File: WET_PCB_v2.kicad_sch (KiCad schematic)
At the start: 0 parts

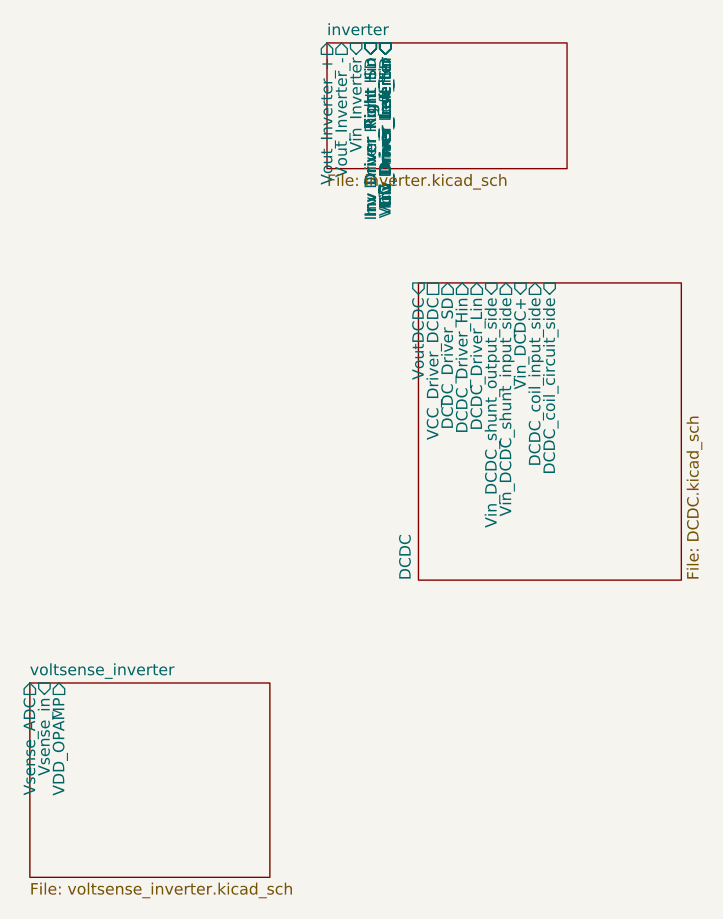
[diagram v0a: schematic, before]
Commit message: Autosave
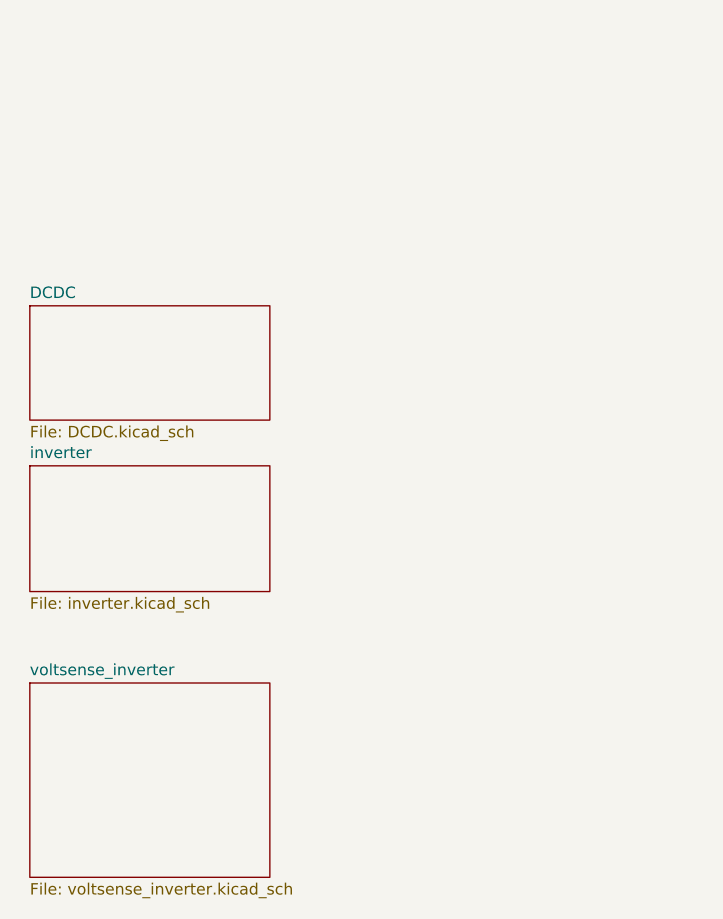
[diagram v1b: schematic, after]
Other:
- sheet DCDC ports: added none; removed DCDC_Driver_Hin, DCDC_Driver_Lin, DCDC_Driver_SD, DCDC_coil_circuit_side, DCDC_coil_input_side, VCC_Driver_DCDC, Vin_DCDC+, Vin_DCDC_shunt_input_side, Vin_DCDC_shunt_output_side, VoutDCDC
- sheet inverter ports: added none; removed Inv_Driver_Left_Hin, Inv_Driver_Left_Lin, Inv_Driver_Left_SD, Inv_Driver_Right_Hin, Inv_Driver_Right_Lin, Inv_Driver_Right_SD, VCC_Driver_Inverter, VDD_Driver_Inverter, Vin_Inverter, Vout_Inverter_+, Vout_Inverter_-
- sheet voltsense_inverter ports: added none; removed VDD_OPAMP, Vsense_ADC, Vsense_in
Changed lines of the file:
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@@
 	(paper "A4")
 	(sheet
-		(at 76.2 68.58)
-		(size 29.21 33.02)
+		(at 33.02 71.12)
+		(size 26.67 12.7)
 		(exclude_from_sim no)
 		(in_bom yes)
@@
 		)
 		(property "Sheetname" "DCDC"
-			(at 75.4884 101.6 90)
+			(at 33.02 70.4084 0)
 			(show_name no)
 			(do_not_autoplace no)
@@
 		)
 		(property "Sheetfile" "DCDC.kicad_sch"
-			(at 105.9946 101.6 90)
+			(at 33.02 84.4046 0)
 			(show_name no)
 			(do_not_autoplace no)
@@
 				)
 				(justify left top)
-			)
-		)
-		(pin "VoutDCDC" input
-			(at 76.2 68.58 90)
-			(effects
-				(font
-					(size 1.27 1.27)
-				)
-				(justify right)
-			)
-		)
-		(pin "VCC_Driver_DCDC" passive
-			(at 77.8193 68.58 90)
-			(effects
-				(font
-					(size 1.27 1.27)
-				)
-				(justify right)
-			)
-		)
-		(pin "DCDC_Driver_SD" output
-			(at 79.4386 68.58 90)
-			(effects
-				(font
-					(size 1.27 1.27)
-				)
-				(justify right)
-			)
-		)
-		(pin "DCDC_Driver_Hin" output
-			(at 81.0579 68.58 90)
-			(effects
-				(font
-					(size 1.27 1.27)
-				)
-				(justify right)
-			)
-		)
-		(pin "DCDC_Driver_Lin" output
-			(at 82.6772 68.58 90)
-			(effects
-				(font
-					(size 1.27 1.27)
-				)
-				(justify right)
-			)
-		)
-		(pin "Vin_DCDC_shunt_output_side" input
-			(at 84.2965 68.58 90)
-			(effects
-				(font
-					(size 1.27 1.27)
-				)
-				(justify right)
-			)
-		)
-		(pin "Vin_DCDC_shunt_input_side" output
-			(at 85.9158 68.58 90)
-			(effects
-				(font
-					(size 1.27 1.27)
-				)
-				(justify right)
-			)
-		)
-		(pin "Vin_DCDC+" input
-			(at 87.5351 68.58 90)
-			(effects
-				(font
-					(size 1.27 1.27)
-				)
-				(justify right)
-			)
-		)
-		(pin "DCDC_coil_input_side" output
-			(at 89.1544 68.58 90)
-			(effects
-				(font
-					(size 1.27 1.27)
-				)
-				(justify right)
-			)
-		)
-		(pin "DCDC_coil_circuit_side" input
-			(at 90.7737 68.58 90)
-			(effects
-				(font
-					(size 1.27 1.27)
-				)
-				(justify right)
 			)
 		)
@@
 			)
 		)
-		(pin "Vsense_ADC" output
-			(at 33.02 113.03 90)
-			(effects
-				(font
-					(size 1.27 1.27)
-				)
-				(justify right)
-			)
-		)
-		(pin "Vsense_in" input
-			(at 34.6393 113.03 90)
-			(effects
-				(font
-					(size 1.27 1.27)
-				)
-				(justify right)
-			)
-		)
-		(pin "VDD_OPAMP" output
-			(at 36.2586 113.03 90)
-			(effects
-				(font
-					(size 1.27 1.27)
-				)
-				(justify right)
-			)
-		)
 		(instances
 			(project "WET_PCB_v2"
@@
 	)
 	(sheet
-		(at 66.04 41.91)
+		(at 33.02 88.9)
 		(size 26.67 13.97)
 		(exclude_from_sim no)
@@
 		)
 		(property "Sheetname" "inverter"
-			(at 66.04 41.1984 0)
+			(at 33.02 88.1884 0)
 			(show_name no)
 			(do_not_autoplace no)
@@
 		)
 		(property "Sheetfile" "inverter.kicad_sch"
-			(at 66.04 56.4646 0)
+			(at 33.02 103.4546 0)
 			(show_name no)
 			(do_not_autoplace no)
@@
 			)
 		)
-		(pin "Vout_Inverter_+" output
-			(at 66.04 41.91 90)
-			(effects
-				(font
-					(size 1.27 1.27)
-				)
-				(justify right)
-			)
-		)
-		(pin "Vout_Inverter_-" output
-			(at 67.6593 41.91 90)
-			(effects
-				(font
-					(size 1.27 1.27)
-				)
-				(justify right)
-			)
-		)
-		(pin "Vin_Inverter" input
-			(at 69.2786 41.91 90)
-			(effects
-				(font
-					(size 1.27 1.27)
-				)
-				(justify right)
-			)
-		)
-		(pin "Inv_Driver_Right_SD" input
-			(at 70.8979 41.91 90)
-			(effects
-				(font
-					(size 1.27 1.27)
-				)
-				(justify right)
-			)
-		)
-		(pin "Inv_Driver_Right_Lin" input
-			(at 70.8979 41.91 90)
-			(effects
-				(font
-					(size 1.27 1.27)
-				)
-				(justify right)
-			)
-		)
-		(pin "Inv_Driver_Right_Hin" input
-			(at 70.8979 41.91 90)
-			(effects
-				(font
-					(size 1.27 1.27)
-				)
-				(justify right)
-			)
-		)
-		(pin "Inv_Driver_Left_SD" input
-			(at 72.5172 41.91 90)
-			(effects
-				(font
-					(size 1.27 1.27)
-				)
-				(justify right)
-			)
-		)
-		(pin "Inv_Driver_Left_Lin" input
-			(at 72.5172 41.91 90)
-			(effects
-				(font
-					(size 1.27 1.27)
-				)
-				(justify right)
-			)
-		)
-		(pin "Inv_Driver_Left_Hin" input
-			(at 72.5172 41.91 90)
-			(effects
-				(font
-					(size 1.27 1.27)
-				)
-				(justify right)
-			)
-		)
-		(pin "VDD_Driver_Inverter" input
-			(at 72.5172 41.91 90)
-			(effects
-				(font
-					(size 1.27 1.27)
-				)
-				(justify right)
-			)
-		)
-		(pin "VCC_Driver_Inverter" input
-			(at 72.5172 41.91 90)
-			(effects
-				(font
-					(size 1.27 1.27)
-				)
-				(justify right)
-			)
-		)

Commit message: Autosave
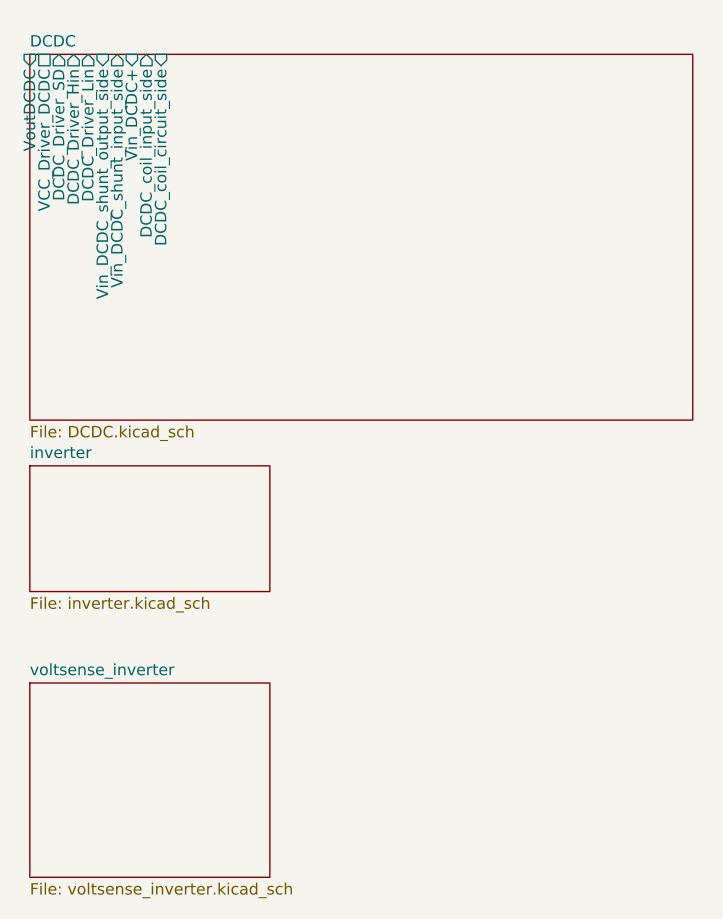
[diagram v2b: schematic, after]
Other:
- sheet DCDC ports: added DCDC_Driver_Hin, DCDC_Driver_Lin, DCDC_Driver_SD, DCDC_coil_circuit_side, DCDC_coil_input_side, VCC_Driver_DCDC, Vin_DCDC+, Vin_DCDC_shunt_input_side, Vin_DCDC_shunt_output_side, VoutDCDC; removed none
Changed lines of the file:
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@@
 	(paper "A4")
 	(sheet
-		(at 33.02 71.12)
-		(size 26.67 12.7)
+		(at 33.02 43.18)
+		(size 73.66 40.64)
 		(exclude_from_sim no)
 		(in_bom yes)
@@
 		)
 		(property "Sheetname" "DCDC"
-			(at 33.02 70.4084 0)
+			(at 33.02 42.4684 0)
 			(show_name no)
 			(do_not_autoplace no)
@@
 			)
 		)
+		(pin "VoutDCDC" input
+			(at 33.02 43.18 90)
+			(effects
+				(font
+					(size 1.27 1.27)
+				)
+				(justify right)
+			)
+		)
+		(pin "VCC_Driver_DCDC" passive
+			(at 34.6393 43.18 90)
+			(effects
+				(font
+					(size 1.27 1.27)
+				)
+				(justify right)
+			)
+		)
+		(pin "DCDC_Driver_SD" output
+			(at 36.2586 43.18 90)
+			(effects
+				(font
+					(size 1.27 1.27)
+				)
+				(justify right)
+			)
+		)
+		(pin "DCDC_Driver_Hin" output
+			(at 37.8779 43.18 90)
+			(effects
+				(font
+					(size 1.27 1.27)
+				)
+				(justify right)
+			)
+		)
+		(pin "DCDC_Driver_Lin" output
+			(at 39.4972 43.18 90)
+			(effects
+				(font
+					(size 1.27 1.27)
+				)
+				(justify right)
+			)
+		)
+		(pin "Vin_DCDC_shunt_output_side" input
+			(at 41.1165 43.18 90)
+			(effects
+				(font
+					(size 1.27 1.27)
+				)
+				(justify right)
+			)
+		)
+		(pin "Vin_DCDC_shunt_input_side" output
+			(at 42.7358 43.18 90)
+			(effects
+				(font
+					(size 1.27 1.27)
+				)
+				(justify right)
+			)
+		)
+		(pin "Vin_DCDC+" input
+			(at 44.3551 43.18 90)
+			(effects
+				(font
+					(size 1.27 1.27)
+				)
+				(justify right)
+			)
+		)
+		(pin "DCDC_coil_input_side" output
+			(at 45.9744 43.18 90)
+			(effects
+				(font
+					(size 1.27 1.27)
+				)
+				(justify right)
+			)
+		)
+		(pin "DCDC_coil_circuit_side" input
+			(at 47.5937 43.18 90)
+			(effects
+				(font
+					(size 1.27 1.27)
+				)
+				(justify right)
+			)
+		)

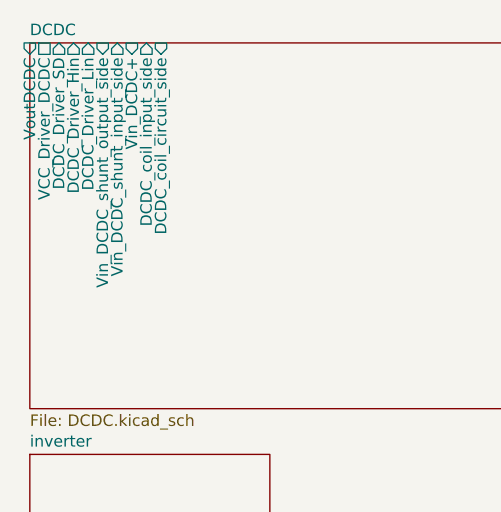
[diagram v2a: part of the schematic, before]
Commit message: Autosave
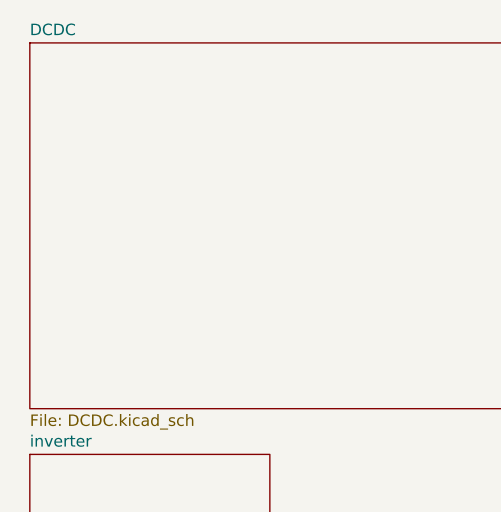
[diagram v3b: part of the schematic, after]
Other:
- sheet DCDC ports: added none; removed DCDC_Driver_Hin, DCDC_Driver_Lin, DCDC_Driver_SD, DCDC_coil_circuit_side, DCDC_coil_input_side, VCC_Driver_DCDC, Vin_DCDC+, Vin_DCDC_shunt_input_side, Vin_DCDC_shunt_output_side, VoutDCDC
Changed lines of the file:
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@@
-			)
-		)
-		(pin "VoutDCDC" input
-			(at 33.02 43.18 90)
-			(effects
-				(font
-					(size 1.27 1.27)
-				)
-				(justify right)
-			)
-		)
-		(pin "VCC_Driver_DCDC" passive
-			(at 34.6393 43.18 90)
-			(effects
-				(font
-					(size 1.27 1.27)
-				)
-				(justify right)
-			)
-		)
-		(pin "DCDC_Driver_SD" output
-			(at 36.2586 43.18 90)
-			(effects
-				(font
-					(size 1.27 1.27)
-				)
-				(justify right)
-			)
-		)
-		(pin "DCDC_Driver_Hin" output
-			(at 37.8779 43.18 90)
-			(effects
-				(font
-					(size 1.27 1.27)
-				)
-				(justify right)
-			)
-		)
-		(pin "DCDC_Driver_Lin" output
-			(at 39.4972 43.18 90)
-			(effects
-				(font
-					(size 1.27 1.27)
-				)
-				(justify right)
-			)
-		)
-		(pin "Vin_DCDC_shunt_output_side" input
-			(at 41.1165 43.18 90)
-			(effects
-				(font
-					(size 1.27 1.27)
-				)
-				(justify right)
-			)
-		)
-		(pin "Vin_DCDC_shunt_input_side" output
-			(at 42.7358 43.18 90)
-			(effects
-				(font
-					(size 1.27 1.27)
-				)
-				(justify right)
-			)
-		)
-		(pin "Vin_DCDC+" input
-			(at 44.3551 43.18 90)
-			(effects
-				(font
-					(size 1.27 1.27)
-				)
-				(justify right)
-			)
-		)
-		(pin "DCDC_coil_input_side" output
-			(at 45.9744 43.18 90)
-			(effects
-				(font
-					(size 1.27 1.27)
-				)
-				(justify right)
-			)
-		)
-		(pin "DCDC_coil_circuit_side" input
-			(at 47.5937 43.18 90)
-			(effects
-				(font
-					(size 1.27 1.27)
-				)
-				(justify right)
 			)
 		)
